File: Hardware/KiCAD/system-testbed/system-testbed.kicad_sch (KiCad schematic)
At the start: 8 parts, among them J2 Stemma QT, J3 Stemma QT, X4 EYESPI, X5 EYESPI

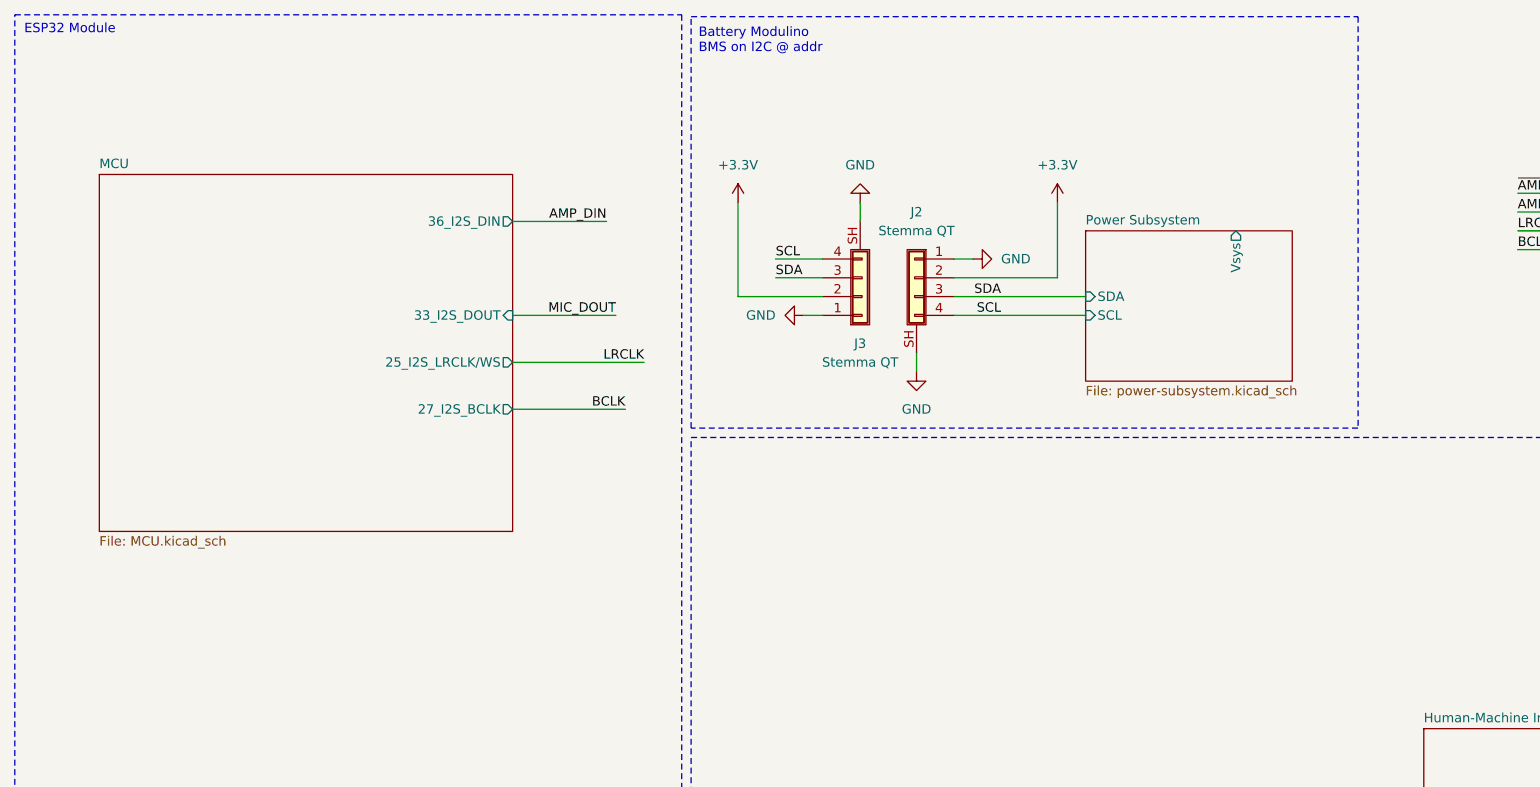
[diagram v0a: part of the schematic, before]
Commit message: feat: schematic capture #63
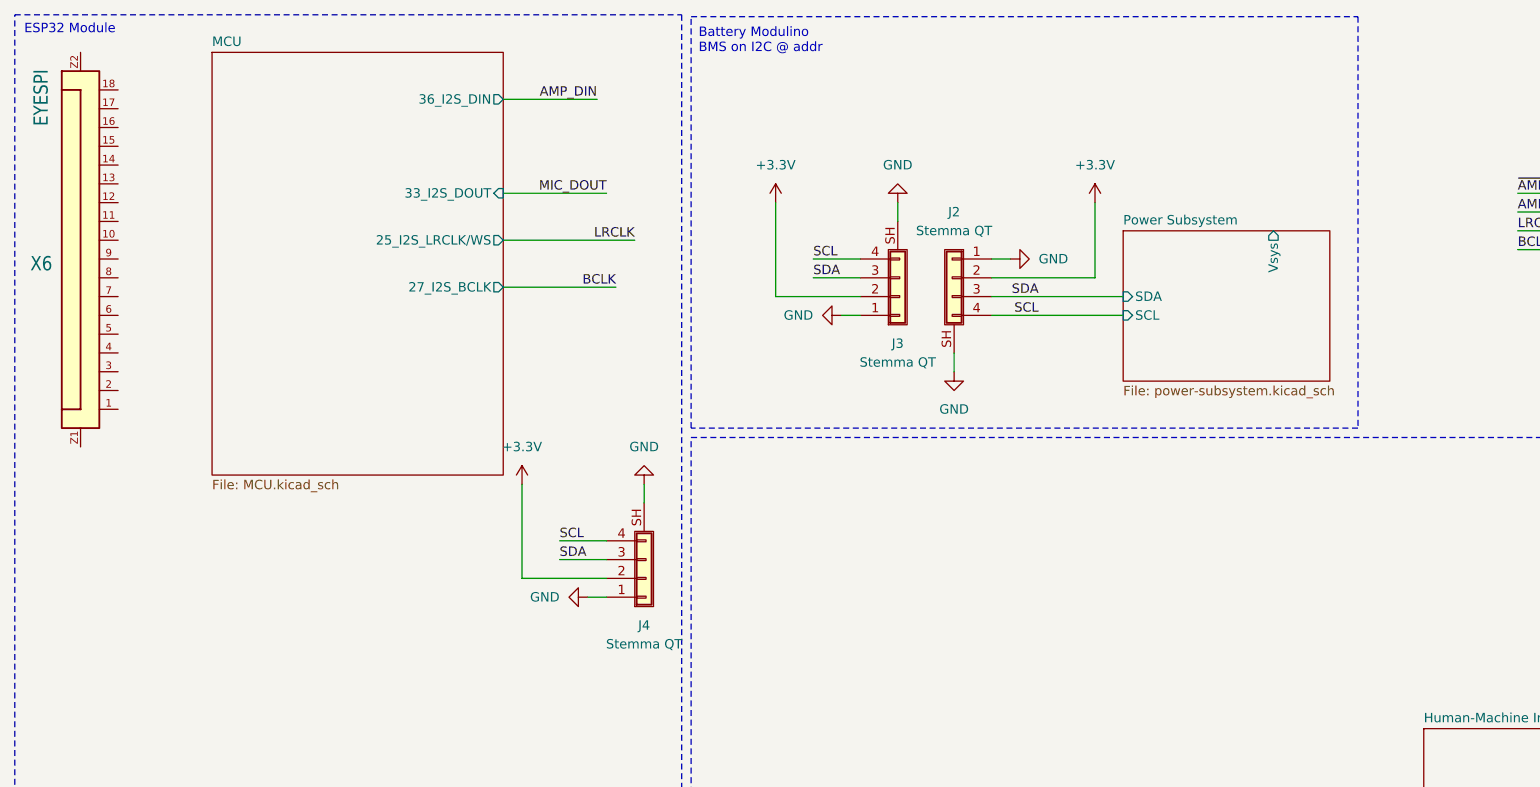
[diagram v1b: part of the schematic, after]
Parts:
- added J4: Stemma QT, Connector_JST:JST_SH_SM04B-SRSS-TB_1x04-1MP_P1.00mm_Horizontal, symbol Connector_Generic_Shielded:Conn_01x04_Shielded
- added X6: EYESPI, capstone-project:Adafruit EYESPI FPC Connector, symbol capstone-project:Adafruit EYESPI FPC Connector
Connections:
- net +3.3V: now also J4.2 (Pin_2)
- net GND: now also J4.1 (Pin_1), J4.SH (Shield)
- net SCL: now also J4.4 (Pin_4)
- net SDA: now also J4.3 (Pin_3)
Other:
- moved on the sheet: J2, J3
